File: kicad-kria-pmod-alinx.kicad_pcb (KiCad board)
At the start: 2 copper layers, 91.4 x 123.2 mm, 35 parts, among them J1 pmod-1, J2 pmod-2, J3 pmod-3, J4 pmod-4, J5 5V, J6 Alinx HDMI/ETH module, J7 ADC module 2-ch, J8 AD DA module, J9 DAC module 2-ch

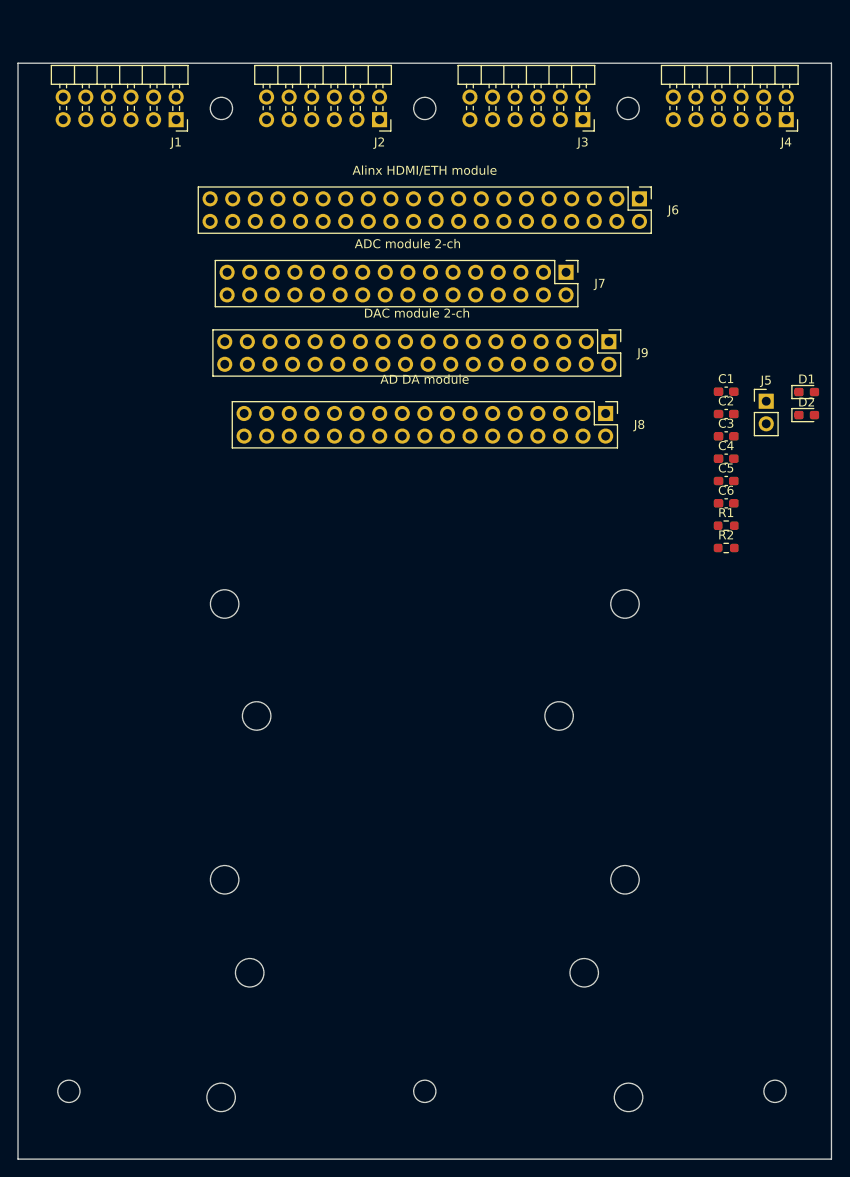
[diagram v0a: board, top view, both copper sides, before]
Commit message: 1.0
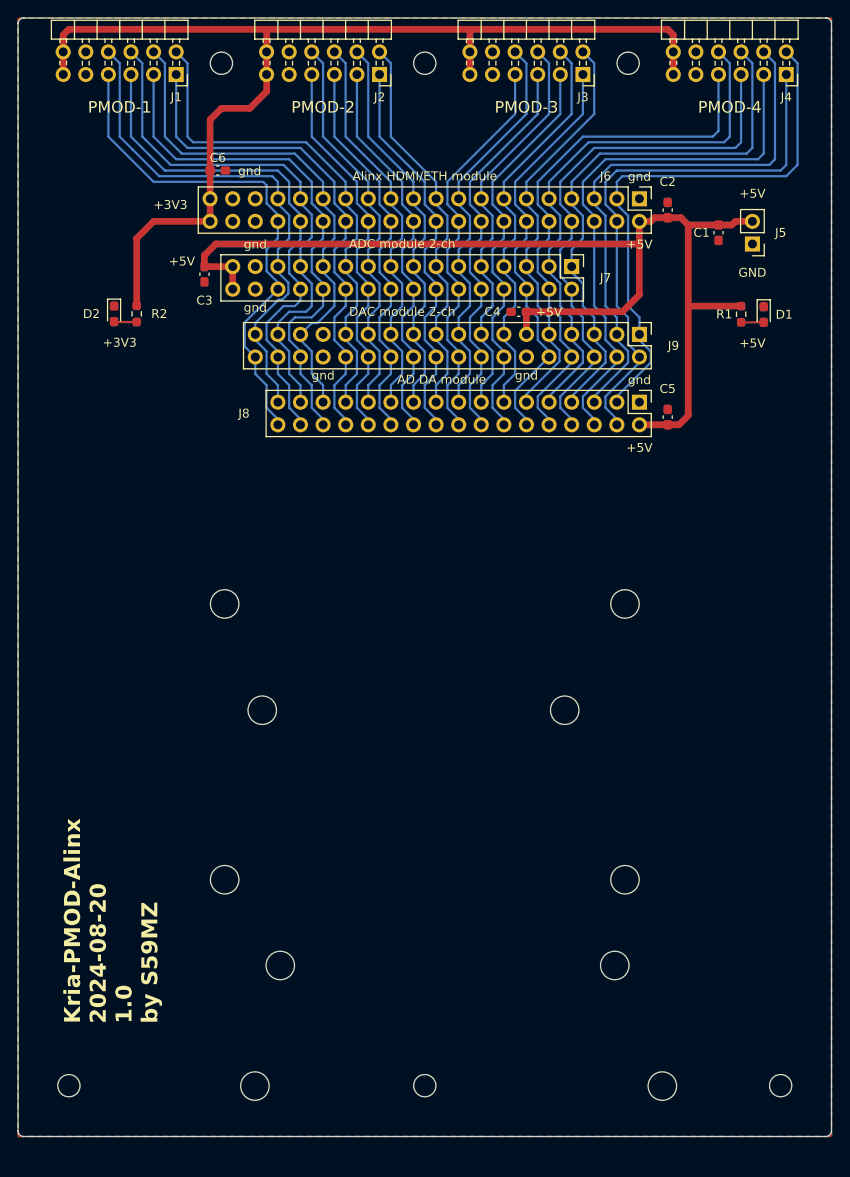
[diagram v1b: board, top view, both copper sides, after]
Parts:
- moved D2 78.7 mm to (81.9, 57.4), turned to -90 degrees
- moved R2 71.3 mm to (84.5, 57.4), turned to -90 degrees
- moved C6 68.3 mm to (93.6, 41.3)
- moved C3 61.4 mm to (92.1, 52.9), turned to -90 degrees
- moved C4 28.6 mm to (127.4, 57.2), turned to 180 degrees
- moved C2 23.8 mm to (144.2, 45.7), turned to 90 degrees
- moved R1 23.8 mm to (152.4, 57.4), turned to -90 degrees
- moved C1 17.9 mm to (149.9, 48.3), turned to -90 degrees
- moved J5 17.7 mm to (153.7, 49.5), turned to 180 degrees
- moved D1 9.96 mm to (154.9, 57.5), turned to -90 degrees
- moved C5 9.74 mm to (144.2, 69.0), turned to 90 degrees
- moved H1 5.08 mm to (94.0, 29.2)
- moved H2 5.08 mm to (116.8, 29.2)
- moved H3 5.08 mm to (139.7, 29.2)
- moved J1 5.08 mm to (88.9, 30.5)
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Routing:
- net +5V: track 0.00 -> 127.3 mm
- net +3.3V: track 0.00 -> 125.8 mm
- net /ac12: track 0.00 -> 62.5 mm
- net /ad11: track 0.00 -> 62.3 mm
- net /aa11: track 0.00 -> 62.2 mm
- net /ae10: track 0.00 -> 62.1 mm
- net /aa10: track 0.00 -> 62.1 mm
- net /ad10: track 0.00 -> 61.9 mm
- net /ad12: track 0.00 -> 61.5 mm
- net /af10: track 0.00 -> 61.1 mm
- net /e10: track 0.00 -> 60.0 mm
- net /d11: track 0.00 -> 60.0 mm
- net /d10: track 0.00 -> 59.7 mm
- net /e12: track 0.00 -> 59.3 mm
- net /b11: track 0.00 -> 59.1 mm
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- added copper zone on B.Cu, net GND
- added copper zone on F.Cu, net GND
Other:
- board size 91.4 x 123.2 mm -> 91.4 x 125.7 mm
- board text added: "+3V3"
- board text added: "+5V"
- board text added: "GND"
- board text added: "Kria-PMOD-Alinx 2024-08-20 1.0 by S59MZ"
- board text added: "PMOD-1"
- board text added: "PMOD-2"
- board text added: "PMOD-3"
- board text added: "PMOD-4"
- board text added: "gnd"
